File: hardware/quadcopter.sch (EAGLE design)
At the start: 101 parts, among them J1 AVR_SPI_PRG_6NS, J2 HEADER-0.1IN-2POS-MALE, J3 FTDI_BASICPTH, J5 HEADER-4POS-0.1IN-FEMALE, J6 HEADER-0.1IN-2POS-FEMALE, J7 HEADER-0.1IN-2POS-FEMALE, Q1 MOSFET-VISHAY-SOT23-N-MOSFET, Q2 MOSFET-VISHAY-SOT23-N-MOSFET, Q3 MOSFET-VISHAY-SOT23-N-MOSFET, Q4 MOSFET-VISHAY-SOT23-N-MOSFET, Q5 MOSFET-VISHAY-SOT23-N-MOSFET, Q6 MOSFET-VISHAY-SOT23-N-MOSFET, U1 ATMEGA128RFA1, U2 IMU_LSM-ST-LSM9DS1-IMU-LGA, U3 MOTOR_PADS-MOLEX-0530470210, U4 MOTOR_PADS-MOLEX-0530470210, U5 MOTOR_PADS-MOLEX-0530470210, U6 MOTOR_PADS-MOLEX-0530470210, U7 3.3V, U8 NET_BRIDGE-BRIDGE-SMD, Y1 CRYSTAL5X3

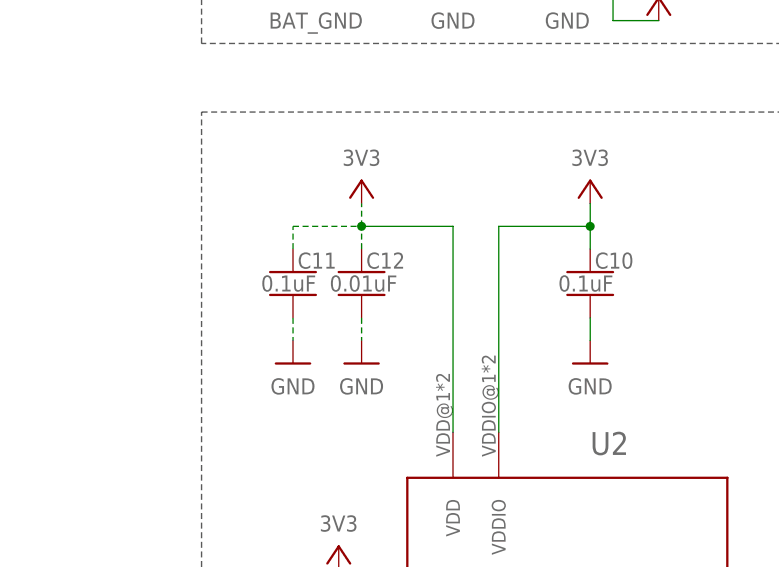
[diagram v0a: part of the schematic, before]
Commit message: Add files via upload
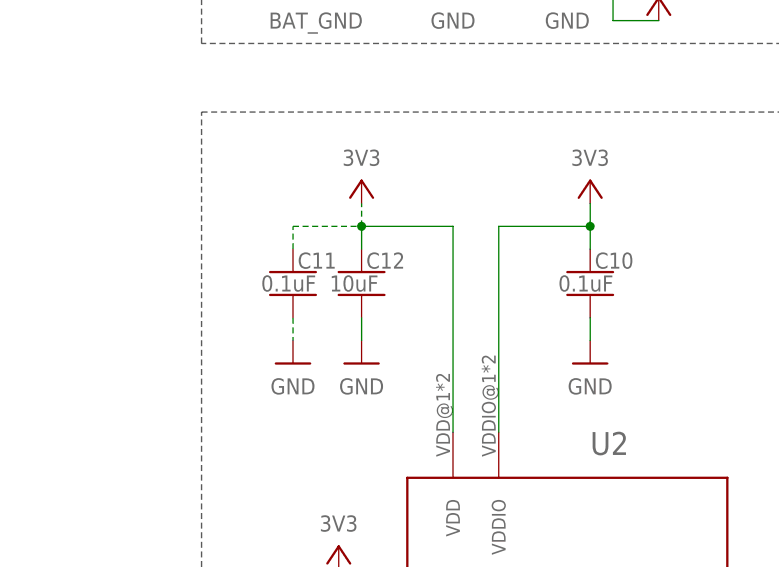
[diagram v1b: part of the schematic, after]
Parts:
- C12: value 0.01uF -> 10uF; device quadparts_prebuilt:CAPACITOR-NP_SMD-2012-0805_CERAMIC-0.01UF -> quadparts_prebuilt:CAPACITOR-NP_SMD-2012-0805_CERAMIC-10UF
